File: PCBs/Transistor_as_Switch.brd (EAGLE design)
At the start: 30 x 20 mm, 7 parts, among them T1 2N3904

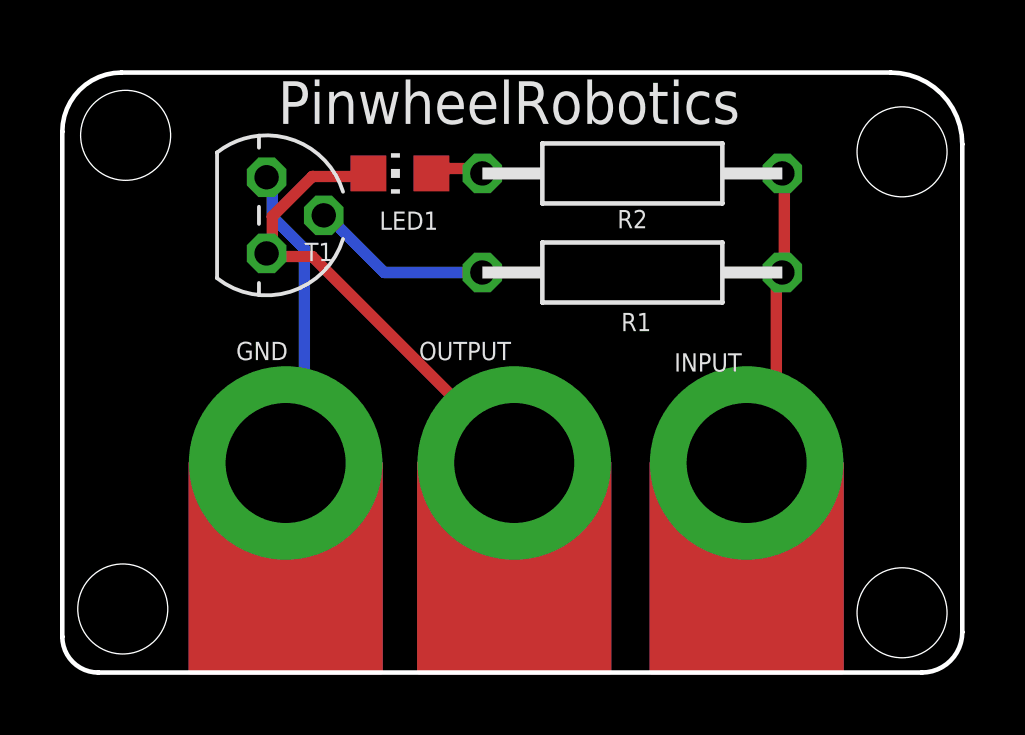
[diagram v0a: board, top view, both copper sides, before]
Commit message: New Update
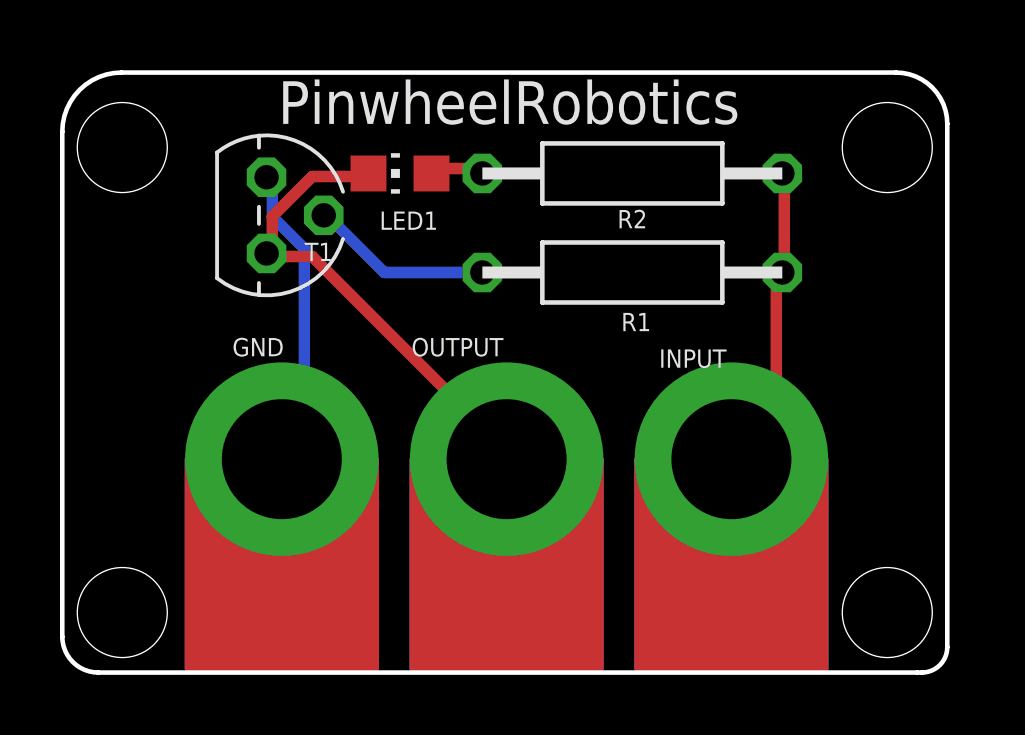
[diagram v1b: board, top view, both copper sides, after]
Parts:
- moved INPUT 0.52 mm to (19.3, 7.11)
- moved OUTPUT 0.28 mm to (11.8, 7.11)
- moved GND 0.18 mm to (4.32, 7.11)
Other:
- board size 30 x 20 mm -> 29.5 x 20 mm
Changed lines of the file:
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@@
 <drawing>
 <settings>
-<setting alwaysvectorfont="no"/>
+<setting alwaysvectorfont="yes"/>
 <setting verticaltext="up"/>
 </settings>
@@
 <board>
 <plain>
-<wire x1="24.612559375" y1="20" x2="-1.0266875" y2="20" width="0.1524" layer="20"/>
+<wire x1="-1.0266875" y1="20" x2="24.792896875" y2="20" width="0.1524" layer="20"/>
+<wire x1="24.792896875" y1="20" x2="26.5" y2="18.292896875" width="0.1524" layer="20" curve="-90"/>
+<wire x1="26.5" y1="18.292896875" x2="26.5" y2="0.845740625" width="0.1524" layer="20"/>
+<wire x1="26.5" y1="0.845740625" x2="25.654259375" y2="0" width="0.1524" layer="20" curve="-90"/>
 <wire x1="-1.0266875" y1="20" x2="-3" y2="18.0266875" width="0.1524" layer="20" curve="90"/>
 <wire x1="-3" y1="18.0266875" x2="-3" y2="1.197415625" width="0.1524" layer="20"/>
 <wire x1="-3" y1="1.197415625" x2="-1.802584375" y2="0" width="0.1524" layer="20" curve="90"/>
-<wire x1="-1.802584375" y1="0" x2="25.654259375" y2="0" width="0.1524" layer="20"/>
-<wire x1="25.654259375" y1="0" x2="27" y2="1.345740625" width="0.1524" layer="20" curve="90"/>
-<wire x1="27" y1="1.345740625" x2="27" y2="17.612559375" width="0.1524" layer="20"/>
-<wire x1="27" y1="17.612559375" x2="24.612559375" y2="20" width="0.1524" layer="20" curve="90"/>
-<hole x="-0.889" y="17.907" drill="3"/>
-<hole x="24.992" y="17.357" drill="3"/>
-<hole x="24.992" y="1.992" drill="3"/>
-<hole x="-0.984" y="2.119" drill="3"/>
+<wire x1="-1.802584375" y1="0" x2="25.5" y2="0" width="0.1524" layer="20"/>
+<hole x="-1" y="17.5" drill="3"/>
+<hole x="24.5" y="17.5" drill="3"/>
+<hole x="24.5" y="2" drill="3"/>
+<hole x="-1" y="2" drill="3"/>
 <text x="4.191" y="18.288" size="1.4224" layer="21">PinwheelRobotics</text>
 <text x="5.461" y="11.811" size="1.27" layer="22" rot="MR180">care@pinwheel.in</text>
+<wire x1="25.5" y1="0" x2="25.654259375" y2="0" width="0.1524" layer="20"/>
 </plain>
 <attributes>
@@
 </autorouter>
 <elements>
-<element name="GND" library="microbit" package="MICROBIT_PAD" value="MICROBIT_PAD" x="4.445" y="6.985" smashed="yes">
-<attribute name="NAME" x="2.794" y="10.414" size="0.6096" layer="21" font="vector"/>
-</element>
-<element name="INPUT" library="microbit" package="MICROBIT_PAD" value="MICROBIT_PAD" x="19.812" y="6.985" smashed="yes">
-<attribute name="NAME" x="17.399" y="10.033" size="0.6096" layer="21" font="vector"/>
+<element name="GND" library="microbit" package="MICROBIT_PAD" value="MICROBIT_PAD" x="4.318" y="7.112" smashed="yes">
+<attribute name="NAME" x="2.667" y="10.541" size="0.6096" layer="21" font="vector"/>
+</element>
+<element name="INPUT" library="microbit" package="MICROBIT_PAD" value="MICROBIT_PAD" x="19.304" y="7.112" smashed="yes">
+<attribute name="NAME" x="16.891" y="10.16" size="0.6096" layer="21" font="vector"/>
 </element>
 <element name="LED1" library="led" library_urn="urn:adsk.eagle:library:259" package="CHIP-LED0805" package3d_urn="urn:adsk.eagle:package:15818/2" value="" x="8.255" y="16.637" smashed="yes" rot="R90">
@@
 <attribute name="VALUE" x="9.525" y="19.177" size="1.27" layer="27" rot="R180"/>
 </element>
-<element name="OUTPUT" library="microbit" package="MICROBIT_PAD" value="MICROBIT_PAD" x="12.065" y="6.985" smashed="yes">
-<attribute name="NAME" x="8.89" y="10.414" size="0.6096" layer="21" font="vector"/>
+<element name="OUTPUT" library="microbit" package="MICROBIT_PAD" value="MICROBIT_PAD" x="11.811" y="7.112" smashed="yes">
+<attribute name="NAME" x="8.636" y="10.541" size="0.6096" layer="21" font="vector"/>
 </element>
 <element name="R1" library="we-rcl" package="R0207/10" value="" x="16.002" y="13.335" smashed="yes" rot="R180">
@@
 <wire x1="21.0693" y1="13.335" x2="21.002" y2="13.335" width="0.381" layer="1"/>
 <wire x1="21.0693" y1="16.5354" x2="21.002" y2="16.637" width="0.381" layer="1"/>
-<wire x1="20.8026" y1="8.001" x2="20.8026" y2="13.335" width="0.381" layer="1"/>
-<wire x1="20.0025" y1="7.2009" x2="20.8026" y2="8.001" width="0.381" layer="1"/>
+<wire x1="20.8026" y1="8.43429375" x2="20.8026" y2="13.335" width="0.381" layer="1"/>
 <wire x1="20.8026" y1="13.335" x2="21.002" y2="13.335" width="0.381" layer="1"/>
-<wire x1="20.0025" y1="7.2009" x2="19.812" y2="6.985" width="0.381" layer="1"/>
+<wire x1="20.8026" y1="8.43429375" x2="19.304" y2="7.112" width="0.381" layer="1"/>
 </signal>
 <signal name="N$1">
@@
 <wire x1="4.0005" y1="14.1351" x2="3.81" y2="13.97" width="0.381" layer="1"/>
 <wire x1="5.334" y1="13.8684" x2="4.0005" y2="13.8684" width="0.381" layer="1"/>
-<wire x1="12.0015" y1="7.2009" x2="5.334" y2="13.8684" width="0.381" layer="1"/>
+<wire x1="11.694584375" y1="7.507815625" x2="5.334" y2="13.8684" width="0.381" layer="1"/>
 <wire x1="4.0005" y1="13.8684" x2="3.81" y2="13.97" width="0.381" layer="1"/>
-<wire x1="12.0015" y1="7.2009" x2="12.065" y2="6.985" width="0.381" layer="1"/>
+<wire x1="11.694584375" y1="7.507815625" x2="11.811" y2="7.112" width="0.381" layer="1"/>
 </signal>
 <signal name="GND">
@@
 <wire x1="4.5339" y1="7.2009" x2="5.0673" y2="7.7343" width="0.381" layer="16"/>
 <wire x1="4.0005" y1="16.2687" x2="3.81" y2="16.51" width="0.381" layer="16"/>
-<wire x1="4.5339" y1="7.2009" x2="4.445" y2="6.985" width="0.381" layer="16"/>
+<wire x1="4.5339" y1="7.2009" x2="4.318" y2="7.112" width="0.381" layer="16"/>
 </signal>
 <signal name="N$3">
